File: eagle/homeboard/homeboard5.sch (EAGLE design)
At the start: 81 parts, among them IC1 XCF02S, IC2 25LC080SN, Q5 BC848SMD, Q6 BC848SMD, Q7 BC848SMD, Q8 BC848SMD, T1 BSS138, T2 BC848, T3 BSS138, U1 XC3S400TQ144, X1 1503_04, X2 SCART-F

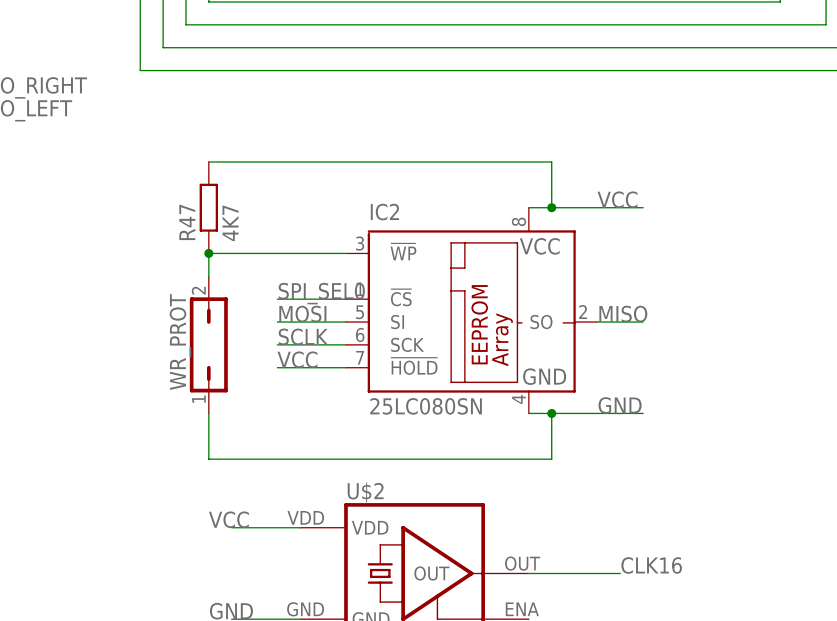
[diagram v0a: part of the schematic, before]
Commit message: rework
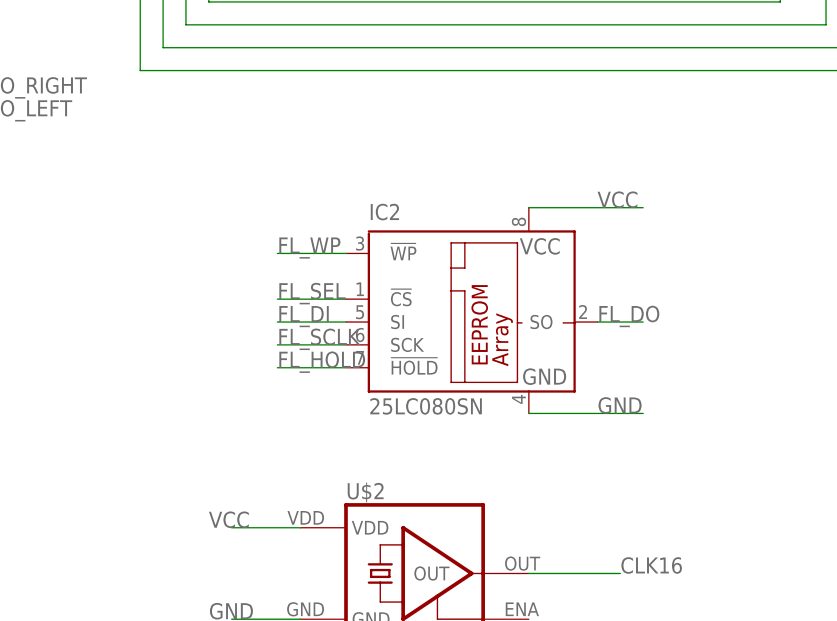
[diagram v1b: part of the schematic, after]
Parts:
- removed R47: 4K7, rcl:R-EU_R0805
- removed WR_PROT: (no value), jumper:JP1Q
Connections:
- net SPI_SEL0 renamed FL_SEL
- removed net N$49: IC2.!WP, R47.1, WR_PROT.2
- new net FL_DI: IC2.SI
- new net FL_DO: IC2.SO
- new net FL_HOLD: IC2.!HOLD
- new net FL_SCLK: IC2.SCK
- new net FL_WP: IC2.!WP
- net GND: no longer WR_PROT.1
- net MISO: no longer IC2.SO
- net MOSI: no longer IC2.SI
- net SCLK: no longer IC2.SCK
- net VCC: no longer IC2.!HOLD, R47.2
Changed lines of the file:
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@@
 <part name="SUPPLY5" library="supply2" deviceset="GND" device=""/>
 <part name="IC2" library="microchip" deviceset="25*" device="SN" technology="LC080"/>
-<part name="R47" library="rcl" deviceset="R-EU_" device="R0805" value="4K7"/>
-<part name="WR_PROT" library="jumper" deviceset="JP1Q" device=""/>
 <part name="R48" library="resistor" deviceset="R-EU_" device="M0805"/>
 <part name="C1" library="resistor" deviceset="C-EU" device="C0603"/>
@@
 <instance part="SUPPLY5" gate="GND" x="83.82" y="17.78"/>
 <instance part="IC2" gate="G$1" x="248.92" y="-78.74"/>
-<instance part="R47" gate="G$1" x="220.98" y="-66.04" rot="R90"/>
-<instance part="WR_PROT" gate="A" x="220.98" y="-81.28"/>
 <instance part="R48" gate="G$1" x="144.78" y="147.32"/>
 <instance part="C1" gate="G$1" x="132.08" y="142.24" rot="R180"/>
@@
 <segment>
 <pinref part="IC2" gate="G$1" pin="GND"/>
-<wire x1="269.24" y1="-88.9" x2="259.08" y2="-88.9" width="0.1524" layer="91"/>
+<wire x1="269.24" y1="-88.9" x2="256.54" y2="-88.9" width="0.1524" layer="91"/>
 <label x="264.16" y="-88.9" size="1.778" layer="95"/>
-<wire x1="259.08" y1="-88.9" x2="256.54" y2="-88.9" width="0.1524" layer="91"/>
-<wire x1="259.08" y1="-88.9" x2="259.08" y2="-93.98" width="0.1524" layer="91"/>
-<junction x="259.08" y="-88.9"/>
-<wire x1="259.08" y1="-93.98" x2="220.98" y2="-93.98" width="0.1524" layer="91"/>
-<pinref part="WR_PROT" gate="A" pin="1"/>
-<wire x1="220.98" y1="-93.98" x2="220.98" y2="-88.9" width="0.1524" layer="91"/>
 </segment>
 <segment>
@@
 <segment>
 <pinref part="IC2" gate="G$1" pin="VCC"/>
-<wire x1="256.54" y1="-66.04" x2="259.08" y2="-66.04" width="0.1524" layer="91"/>
 <label x="264.16" y="-66.04" size="1.778" layer="95"/>
-<pinref part="R47" gate="G$1" pin="2"/>
-<wire x1="259.08" y1="-66.04" x2="269.24" y2="-66.04" width="0.1524" layer="91"/>
-<wire x1="220.98" y1="-60.96" x2="259.08" y2="-60.96" width="0.1524" layer="91"/>
-<wire x1="259.08" y1="-60.96" x2="259.08" y2="-66.04" width="0.1524" layer="91"/>
-<junction x="259.08" y="-66.04"/>
-</segment>
-<segment>
-<pinref part="IC2" gate="G$1" pin="!HOLD"/>
-<label x="228.6" y="-83.82" size="1.778" layer="95"/>
-<wire x1="228.6" y1="-83.82" x2="236.22" y2="-83.82" width="0.1524" layer="91"/>
+<wire x1="256.54" y1="-66.04" x2="269.24" y2="-66.04" width="0.1524" layer="91"/>
 </segment>
 <segment>
@@
 <net name="SCLK" class="0">
 <segment>
-<pinref part="IC2" gate="G$1" pin="SCK"/>
-<wire x1="228.6" y1="-81.28" x2="236.22" y2="-81.28" width="0.1524" layer="91"/>
-<label x="228.6" y="-81.28" size="1.778" layer="95"/>
-</segment>
-<segment>
 <pinref part="U$3" gate="G$1" pin="PB1(SCK)"/>
 <wire x1="-127" y1="-144.78" x2="-134.62" y2="-144.78" width="0.1524" layer="91"/>
@@
 <net name="MOSI" class="0">
 <segment>
-<pinref part="IC2" gate="G$1" pin="SI"/>
-<wire x1="228.6" y1="-78.74" x2="236.22" y2="-78.74" width="0.1524" layer="91"/>
-<label x="228.6" y="-78.74" size="1.778" layer="95"/>
-</segment>
-<segment>
 <pinref part="U$3" gate="G$1" pin="PB2(PDI/MOSI)"/>
 <wire x1="-127" y1="-142.24" x2="-134.62" y2="-142.24" width="0.1524" layer="91"/>
@@
 <net name="MISO" class="0">
 <segment>
-<pinref part="IC2" gate="G$1" pin="SO"/>
-<wire x1="269.24" y1="-78.74" x2="264.16" y2="-78.74" width="0.1524" layer="91"/>
-<label x="264.16" y="-78.74" size="1.778" layer="95"/>
-</segment>
-<segment>
 <pinref part="U$3" gate="G$1" pin="PB3(PDO/MISO)"/>
 <wire x1="-127" y1="-139.7" x2="-134.62" y2="-139.7" width="0.1524" layer="91"/>
@@
 </segment>
 </net>
-<net name="SPI_SEL0" class="0">
+<net name="FL_SEL" class="0">
 <segment>
 <pinref part="IC2" gate="G$1" pin="!CS"/>
 <wire x1="228.6" y1="-76.2" x2="236.22" y2="-76.2" width="0.1524" layer="91"/>
 <label x="228.6" y="-76.2" size="1.778" layer="95"/>
-</segment>
-</net>
-<net name="N$49" class="0">
-<segment>
-<pinref part="IC2" gate="G$1" pin="!WP"/>
-<wire x1="220.98" y1="-71.12" x2="236.22" y2="-71.12" width="0.1524" layer="91"/>
-<pinref part="R47" gate="G$1" pin="1"/>
-<pinref part="WR_PROT" gate="A" pin="2"/>
-<wire x1="220.98" y1="-73.66" x2="220.98" y2="-71.12" width="0.1524" layer="91"/>
-<junction x="220.98" y="-71.12"/>
 </segment>
 </net>
@@
 </segment>
 </net>
+<net name="FL_HOLD" class="0">
+<segment>
+<pinref part="IC2" gate="G$1" pin="!HOLD"/>
+<label x="228.6" y="-83.82" size="1.778" layer="95"/>
+<wire x1="228.6" y1="-83.82" x2="236.22" y2="-83.82" width="0.1524" layer="91"/>
+</segment>
+</net>
+<net name="FL_SCLK" class="0">
+<segment>
+<pinref part="IC2" gate="G$1" pin="SCK"/>
+<wire x1="228.6" y1="-81.28" x2="236.22" y2="-81.28" width="0.1524" layer="91"/>
+<label x="228.6" y="-81.28" size="1.778" layer="95"/>
+</segment>
+</net>
+<net name="FL_DI" class="0">
+<segment>
+<pinref part="IC2" gate="G$1" pin="SI"/>
+<wire x1="228.6" y1="-78.74" x2="236.22" y2="-78.74" width="0.1524" layer="91"/>
+<label x="228.6" y="-78.74" size="1.778" layer="95"/>
+</segment>
+</net>
+<net name="FL_DO" class="0">
+<segment>
+<pinref part="IC2" gate="G$1" pin="SO"/>
+<wire x1="269.24" y1="-78.74" x2="264.16" y2="-78.74" width="0.1524" layer="91"/>
+<label x="264.16" y="-78.74" size="1.778" layer="95"/>
+</segment>
+</net>
+<net name="FL_WP" class="0">
+<segment>
+<pinref part="IC2" gate="G$1" pin="!WP"/>
+<wire x1="228.6" y1="-71.12" x2="236.22" y2="-71.12" width="0.1524" layer="91"/>
+<label x="228.6" y="-71.12" size="1.778" layer="95"/>
+</segment>
+</net>
